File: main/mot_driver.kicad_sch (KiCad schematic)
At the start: 0 parts

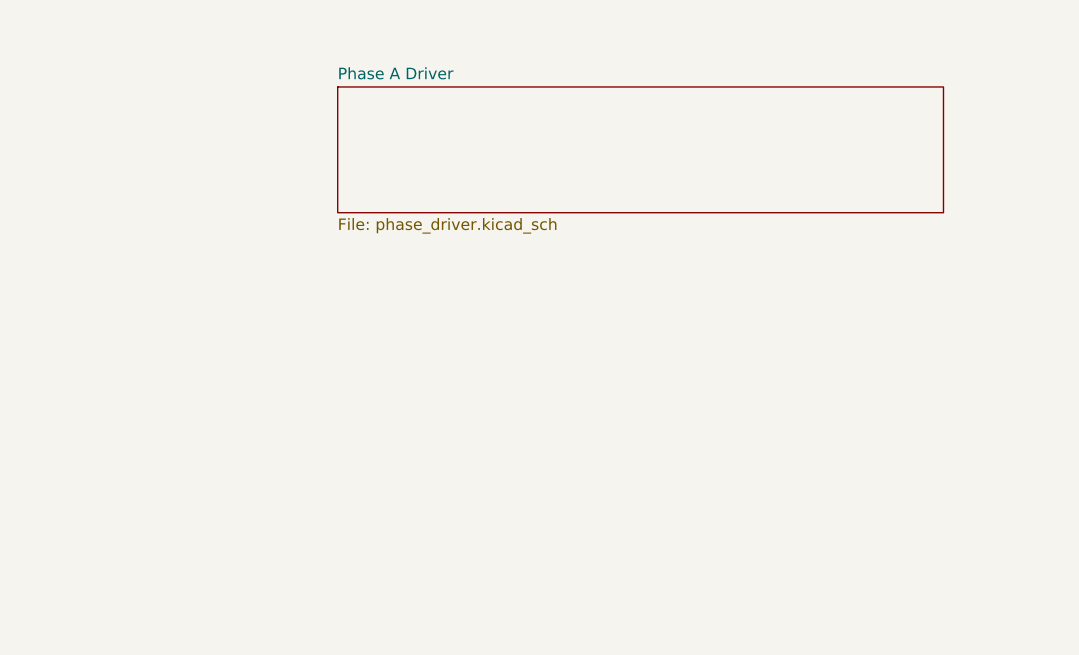
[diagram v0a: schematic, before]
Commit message: PSU should be OK
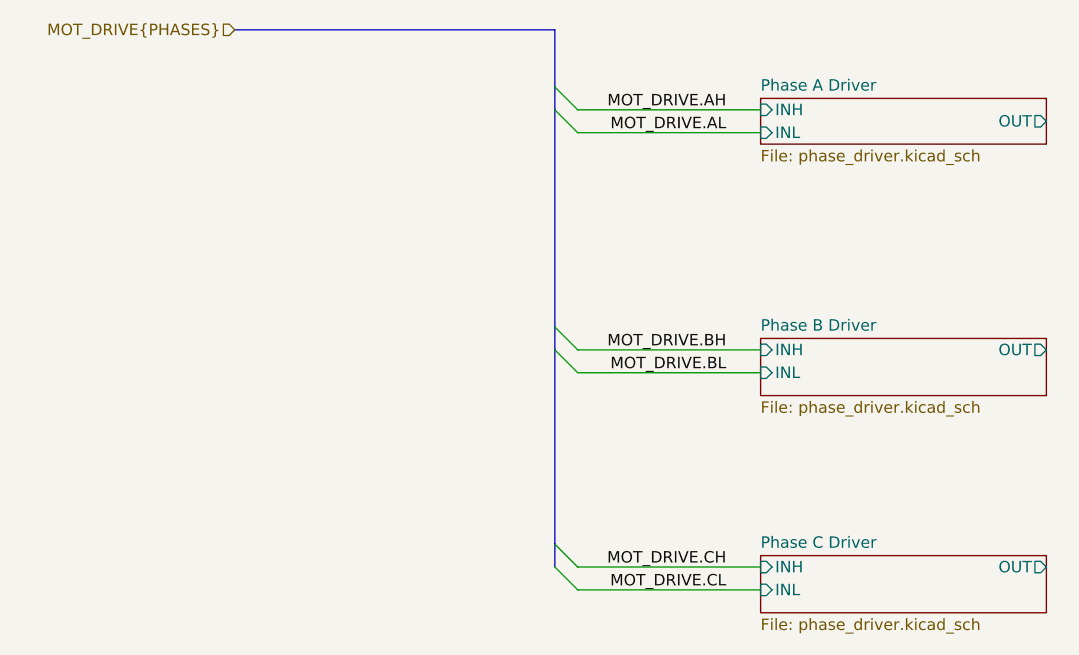
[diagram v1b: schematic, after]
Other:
- added sheet Phase B Driver (phase_driver.kicad_sch)
- added sheet Phase C Driver (phase_driver.kicad_sch)
- sheet Phase A Driver ports: added INH, INL, OUT; removed none
